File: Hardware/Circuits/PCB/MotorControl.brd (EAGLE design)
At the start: 72 x 150 mm, 60 parts, among them U1 LTC4359CMS8PBF

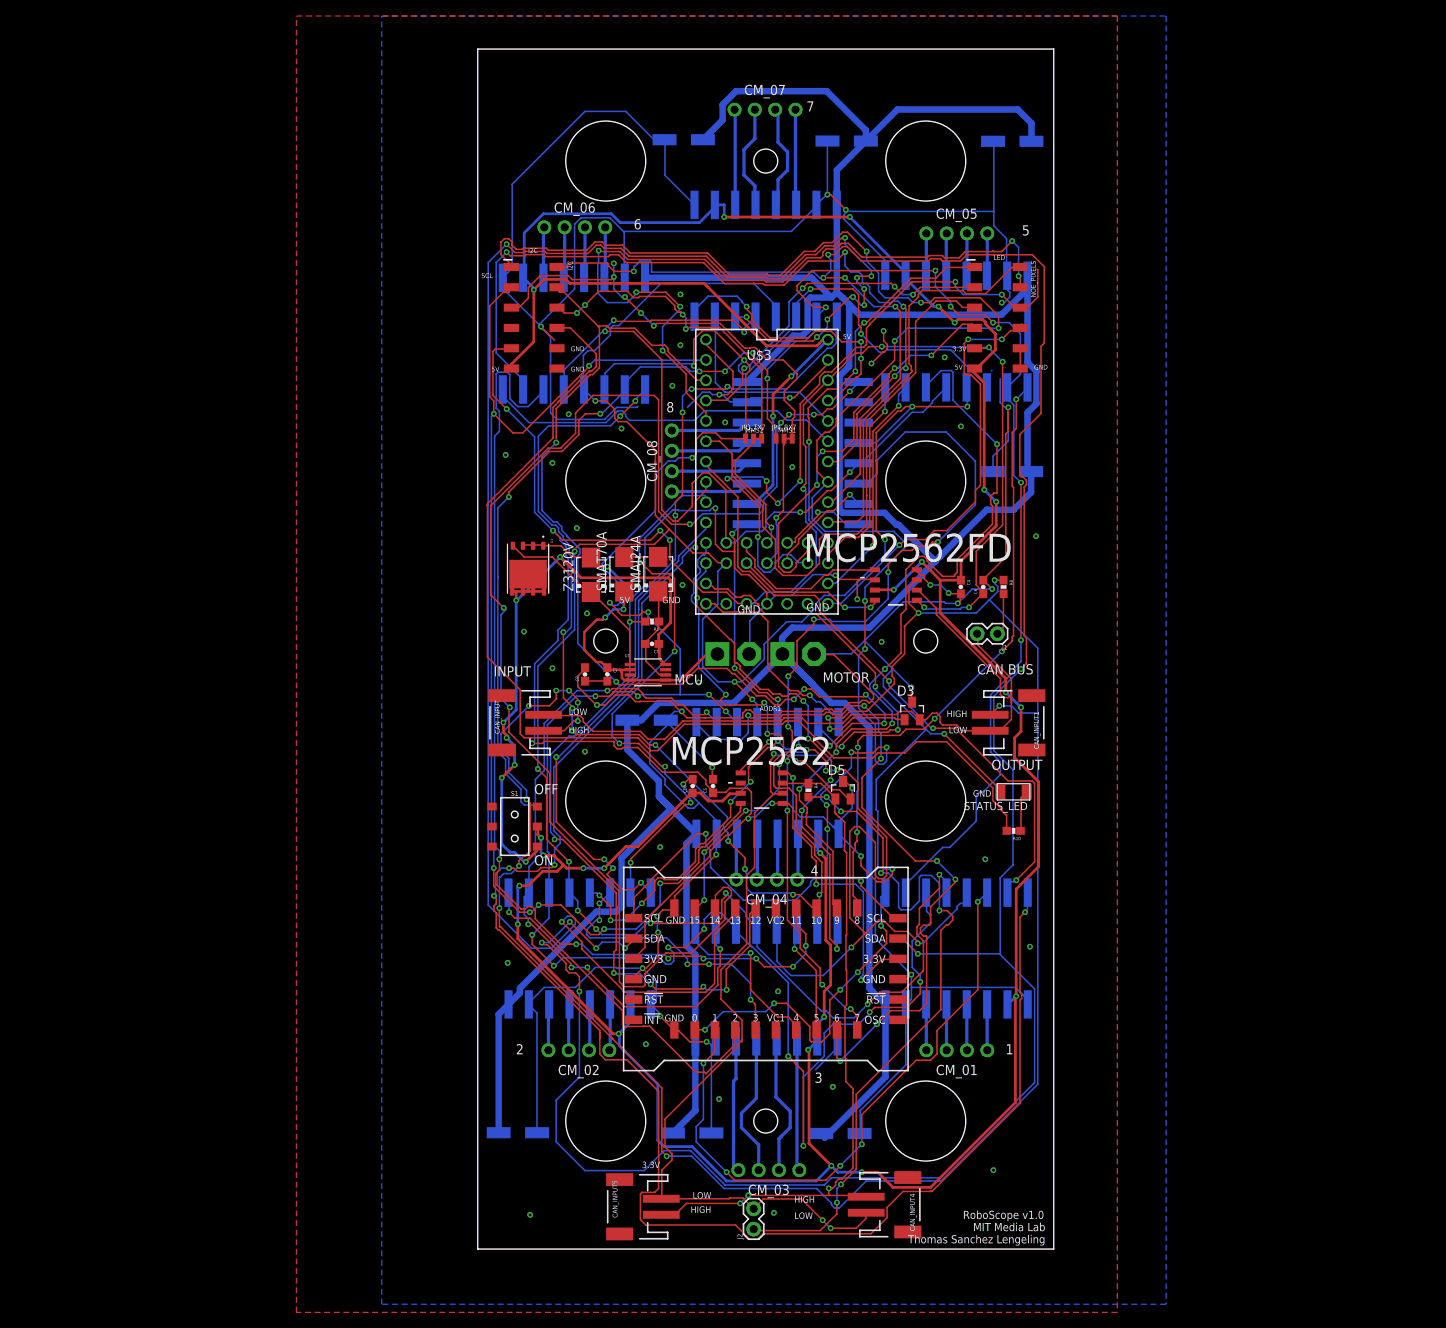
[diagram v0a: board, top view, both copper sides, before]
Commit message: circuits
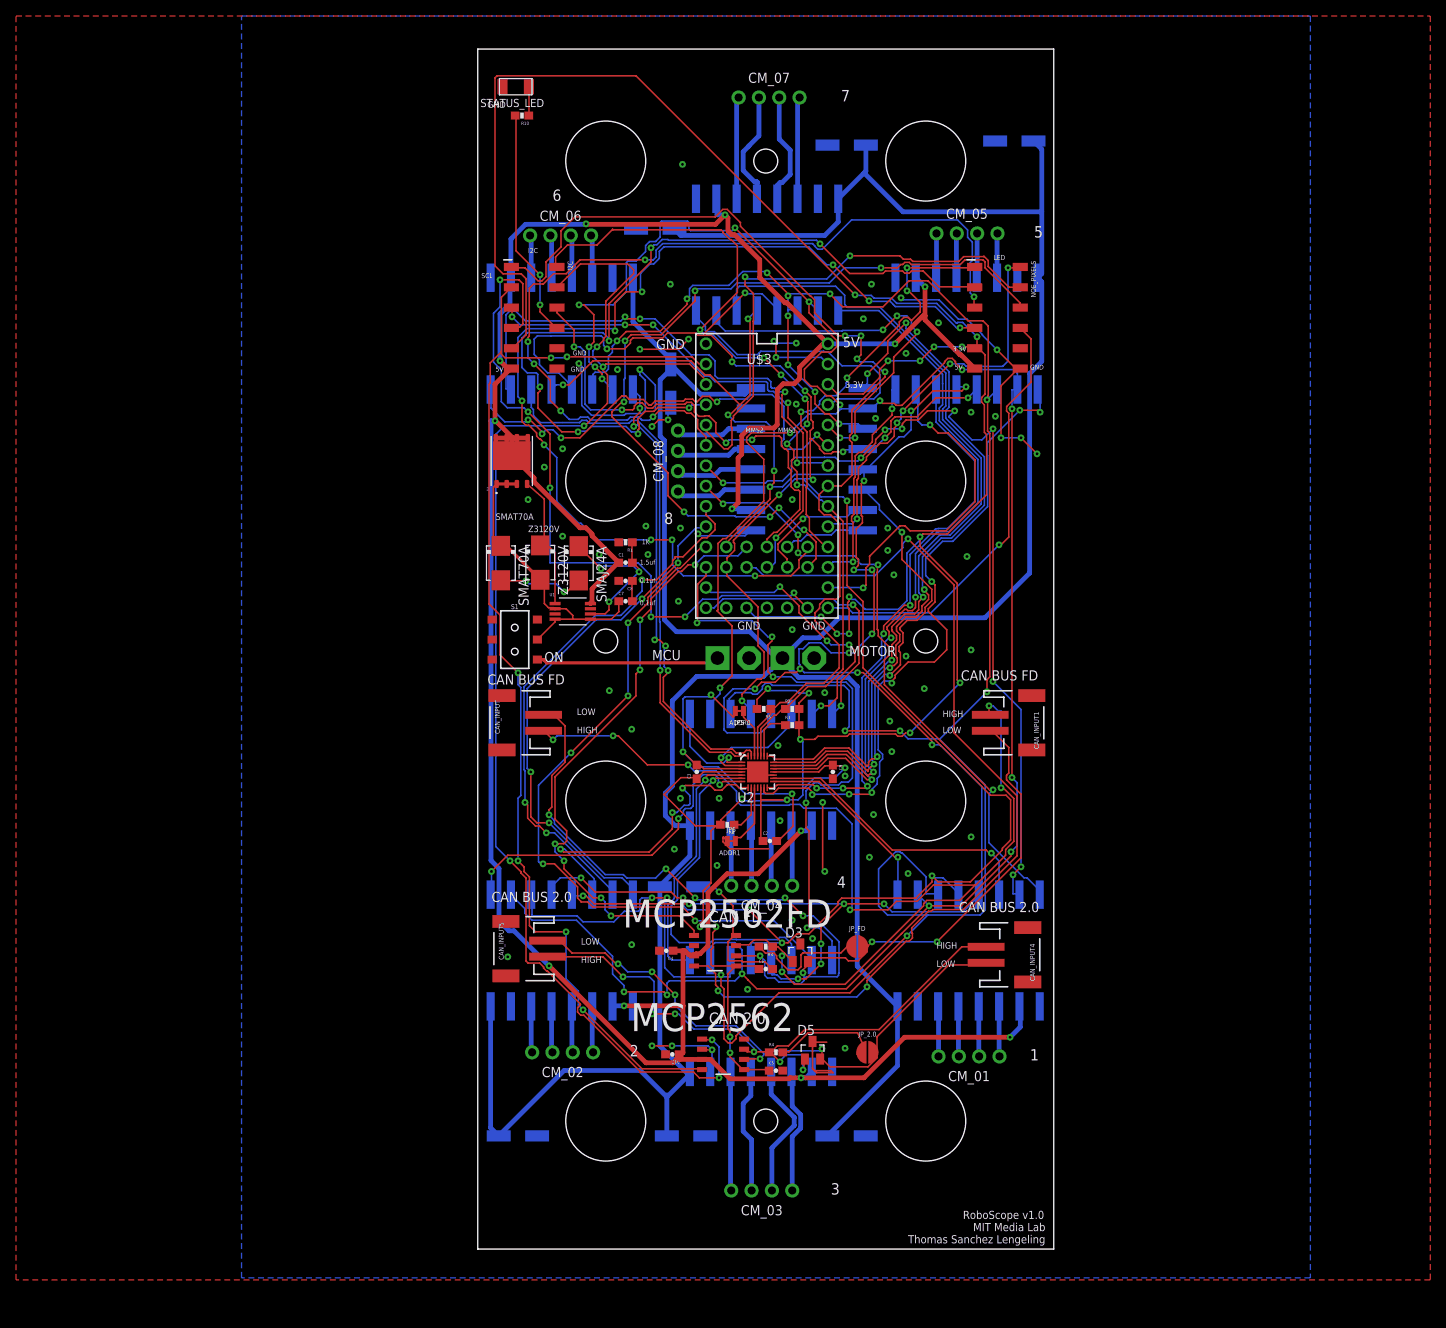
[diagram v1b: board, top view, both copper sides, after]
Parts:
- removed J1, J2: (no value), SparkFun-Connectors:1X02
- removed JP3_TX7, JP4_RX7: JUMPER-SMT_3_1-NC_TRACE_NO-SILK, SparkFun-Jumpers:SMT-JUMPER_3_1-NC_TRACE_NO-SILK
- removed U$5: SX1509, SX1509_s:SX1509
- added C2, C3, C9: 0.1uF, SparkFun-Capacitors:0603-CAP
- added JP5, JP6: JUMPER-SMT_2_NC_TRACE_NO-SILK, SparkFun-Jumpers:SMT-JUMPER_2_NC_TRACE_NO-SILK
- added JP_2.0, JP_FD: JUMPER-SMT_2_NO_NO-SILK_ROUND, SparkFun-Jumpers:SMT-JUMPER_2_NO_NO-SILK_ROUND
- added R2, R3, R5, R6: 10K, SparkFun-Resistors:0603-RES
- added U2: SX1509, SparkFun-DigitalIC:QFN-28
- moved R10 108.5 mm to (7.62, 144.8)
- moved STATUS_LED 107.9 mm to (6.84, 148.4)
- moved C4 58.5 mm to (25.7, 40.4), turned to 180 degrees
- moved C6 54.9 mm to (38.1, 38.1), turned to 0 degrees
- moved R8 53.9 mm to (38.1, 40.9), turned to 180 degrees
- moved MCP2562FD 51.0 mm to (31.8, 40.4)
- moved MC8 44.0 mm to (26.2, 111.3), turned to 90 degrees
- moved C5 36.4 mm to (39.4, 25.4), turned to 0 degrees
- moved CAN_INPUT5 35.3 mm to (7.11, 40.6)
- moved CAN_INPUT4 34.7 mm to (69.3, 39.9)
- moved C10 33.6 mm to (26.4, 27.4), turned to 180 degrees
- moved MCP2562 33.6 mm to (32.8, 27.4)
- moved D3 33.3 mm to (42.4, 40.1)
- moved R4 33.0 mm to (39.4, 27.7), turned to 0 degrees
- moved D5 32.7 mm to (43.9, 27.9)
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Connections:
- removed net 0_SX0: MOTOR_01.ENA, U$5.0
- removed net 10_SX0: MOTOR_06.ENA, U$5.10
- removed net 11_SX0: MOTOR_06.STBY, U$5.11
- removed net 12_SX0: MOTOR_07.ENA, U$5.12
- removed net 13_SX0: MOTOR_07.STBY, U$5.13
- removed net 14_SX0: MOTOR_08.ENA, U$5.14
- removed net 15_SX0: MOTOR_08.STBY, U$5.15
- removed net 1_SX0: MOTOR_01.STBY, U$5.1
- removed net 28_INT_01: JP4_RX7.2, U$3.28
- removed net 29_INT_02: JP3_TX7.2, U$3.29
- removed net 2_SX0: MOTOR_02.ENA, U$5.2
- removed net 3_SX0: MOTOR_02.STBY, U$5.3
- removed net 4_SX0: MOTOR_03.ENA, U$5.4
- removed net 5_SX0: MOTOR_03.STBY, U$5.5
- removed net 6_SX0: MOTOR_04.ENA, U$5.6
- removed net 7_SX0: MOTOR_04.STBY, U$5.7
- removed net 8_SX0: MOTOR_05.ENA, U$5.8
- removed net 9_SX0: MOTOR_05.STBY, U$5.9
- removed net MSS1: MOTOR_08.MS1
- removed net MSS2: MOTOR_08.MS2
- removed net PIN_EX: I2C.7
- removed net REG_5V: C1.1, D1.5, D1.6, D1.7, D1.8, D1.9, S1.3, U1.8
- removed net SCL_00: I2C.1, U$3.19/A5, U$5.SCL, U$5.SCL_2
- removed net SDA_00: I2C.2, U$3.18/A4, U$5.SDA, U$5.SDA_2
- new net !RESET: R3.1, U2.23
- new net OSCIO: U2.11
- new net RESET: I2C.7, U$3.RESET
- new net SX00_!INT: R6.1, U2.9
- new net SX00_0: MOTOR_06.ENA, U2.27
- new net SX00_1: MOTOR_06.STBY, U2.28
- new net SX00_10: MOTOR_01.ENA, U2.15
- new net SX00_11: MOTOR_01.STBY, U2.16
- new net SX00_12: MOTOR_07.ENA, U2.19
- new net SX00_13: MOTOR_07.STBY, U2.20
- new net SX00_14: MOTOR_08.ENA, U2.21
- new net SX00_15: MOTOR_08.STBY, U2.22
- new net SX00_2: MOTOR_04.ENA, U2.1
- new net SX00_3: MOTOR_04.STBY, U2.2
- new net SX00_4: MOTOR_03.ENA, U2.5
- new net SX00_5: MOTOR_03.STBY, U2.6
- new net SX00_6: MOTOR_02.ENA, U2.7
- new net SX00_7: MOTOR_02.STBY, U2.8
- new net SX00_8: MOTOR_05.ENA, U2.13
- new net SX00_9: MOTOR_05.STBY, U2.14
- new net SX00_ADDR0: JP5.1, U2.26
- new net SX00_ADDR1: JP6.2, U2.10
- new net SX00_SCL: I2C.1, R5.1, U$3.19/A5, U2.25
- new net SX00_SDA: I2C.2, R2.1, U$3.18/A4, U2.24
- new net VCC_SWITCH: C7.1, D1.1, D1.2, D1.3, S1.2, SMAT70A.C, U1.2, U1.4, U1.5, Z3120V.A
- net 3.3V: now also C2.1, C3.1, C9.1, R2.2, R3.2, R5.2, R6.2, U2.12, U2.18, U2.4; no longer U$5.3.3V, U$5.3.3V_1
- net CAN_L: now also JP_FD.2; no longer J1.2
- net CAN_L2: now also JP_2.0.2; no longer J2.2
- net GND_MCU: now also C2.2, C3.2, C9.2, JP5.2, JP6.1, U2.17, U2.29, U2.3; no longer U$5.GND, U$5.GND_1, U$5.GND_2, U$5.GND_3
- net INT_01: now also U$3.28; no longer JP4_RX7.3
- net INT_02: now also U$3.29; no longer JP3_TX7.3
- net MMS1: now also MOTOR_08.MS1; no longer JP4_RX7.1
- net MMS2: now also MOTOR_08.MS2; no longer JP3_TX7.1
- net N$1: now also JP_FD.1; no longer J1.1
- net N$3: now also JP_2.0.1; no longer J2.1
- net VCC_5V: now also C1.1, D1.5, D1.6, D1.7, D1.8, D1.9, U1.8; no longer S1.2
- net VCC_MCU: now also S1.3; no longer C7.1, D1.1, D1.2, D1.3, SMAT70A.C, U1.2, U1.4, U1.5, Z3120V.A
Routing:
- net GND_MCU: track 710.2 -> 196.4 mm, vias 66 -> 75
- net SDA_00: track 345.2 -> 0.00 mm, vias 12 -> 0
- net SCL_00: track 239.1 -> 0.00 mm, vias 12 -> 0
- net 13_SX0: track 214.8 -> 0.00 mm, vias 11 -> 0
- net 14_SX0: track 173.1 -> 0.00 mm, vias 7 -> 0
- net 12_SX0: track 136.5 -> 0.00 mm, vias 9 -> 0
- net SX00_SCL: track 0.00 -> 129.5 mm, vias 0 -> 4
- net MDIR_01: track 204.9 -> 78.3 mm
- net 11_SX0: track 126.5 -> 0.00 mm, vias 7 -> 0
- net CAN_H: track 262.8 -> 141.1 mm, vias 14 -> 8
- net SX00_SDA: track 0.00 -> 111.1 mm, vias 0 -> 7
- net SX00_13: track 0.00 -> 109.2 mm, vias 0 -> 3
- net STATUS_PIN: track 134.9 -> 28.8 mm, vias 0 -> 2
- net CAN_RX3: track 18.9 -> 119.8 mm, vias 2 -> 3
- net 10_SX0: track 100.5 -> 0.00 mm, vias 9 -> 0
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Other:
- board text added: "0.1uf"
- board text added: "1.5uf"
- board text added: "1K"
- board text added: "ADDR0"
- board text added: "CAN 2.0"
- board text added: "CAN BUS 2.0"
- board text added: "CAN BUS FD"
- board text added: "CAN FD"
- board text added: "SMAT70A"
- board text added: "Z3120V"
- board text removed: "-"
- board text removed: "CAN BUS"
- board text removed: "INPUT"
- board text removed: "OFF"
- board text removed: "OUTPUT"
